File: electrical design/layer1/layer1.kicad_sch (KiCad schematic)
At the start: 76 parts, among them SW1 SW_DPDT_x2, U1 STM32F103C8T6, U2 CD74HC4067SM, U3 CD74HC4067SM

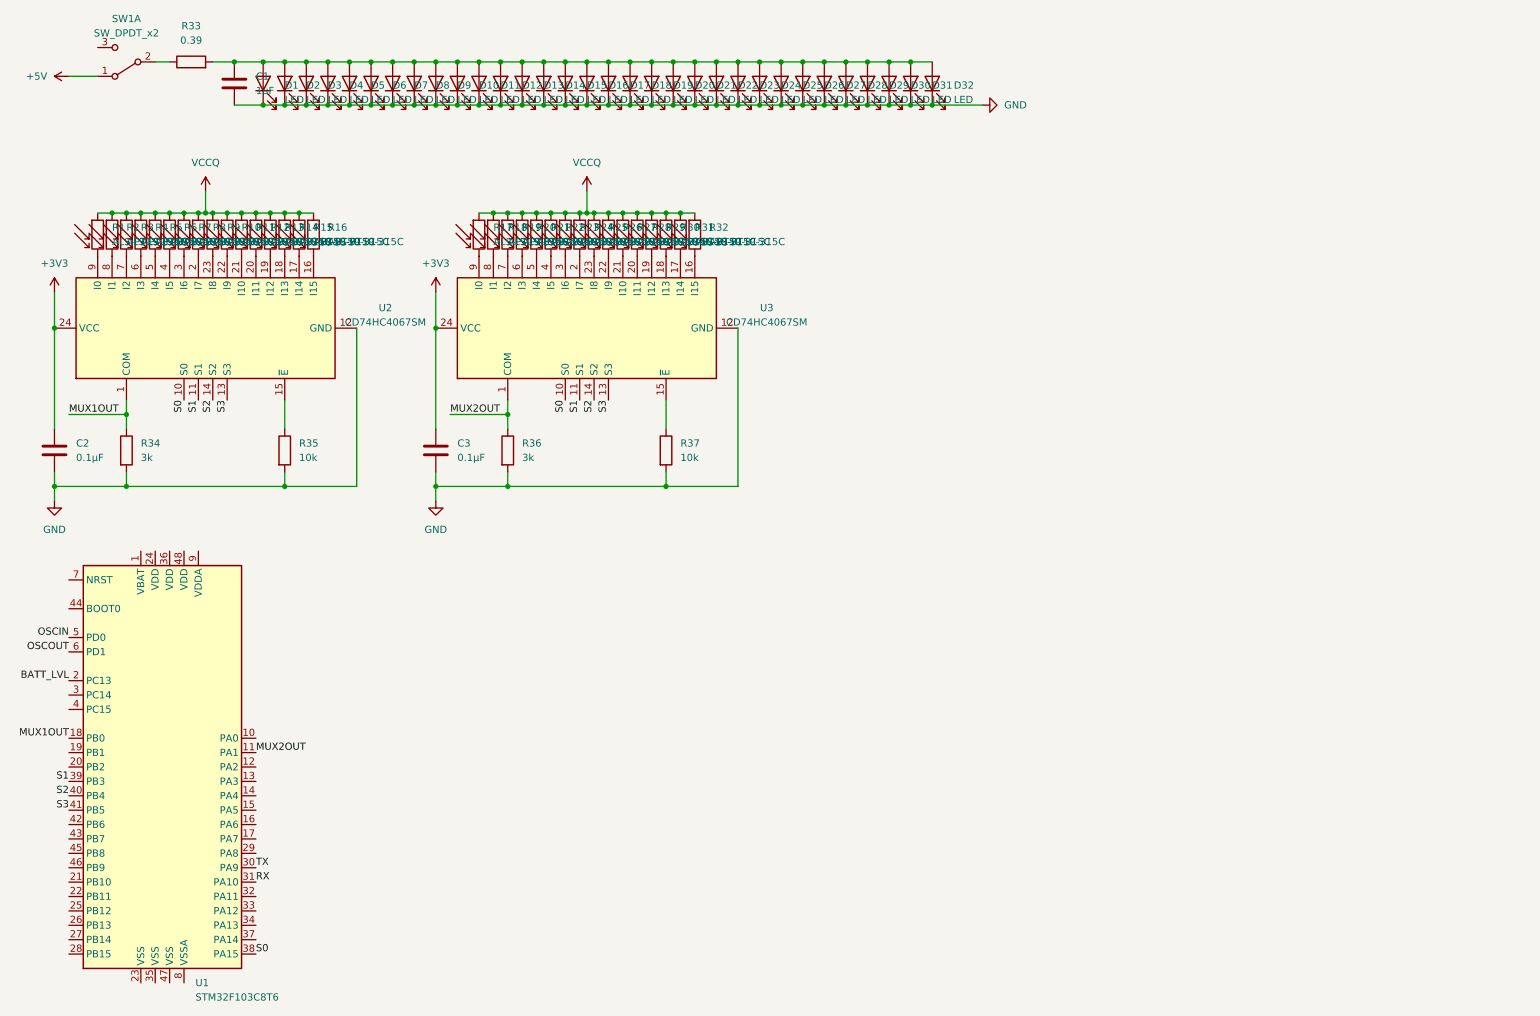
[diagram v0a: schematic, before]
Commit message: finish stm32f103c8t6 sub-circuit
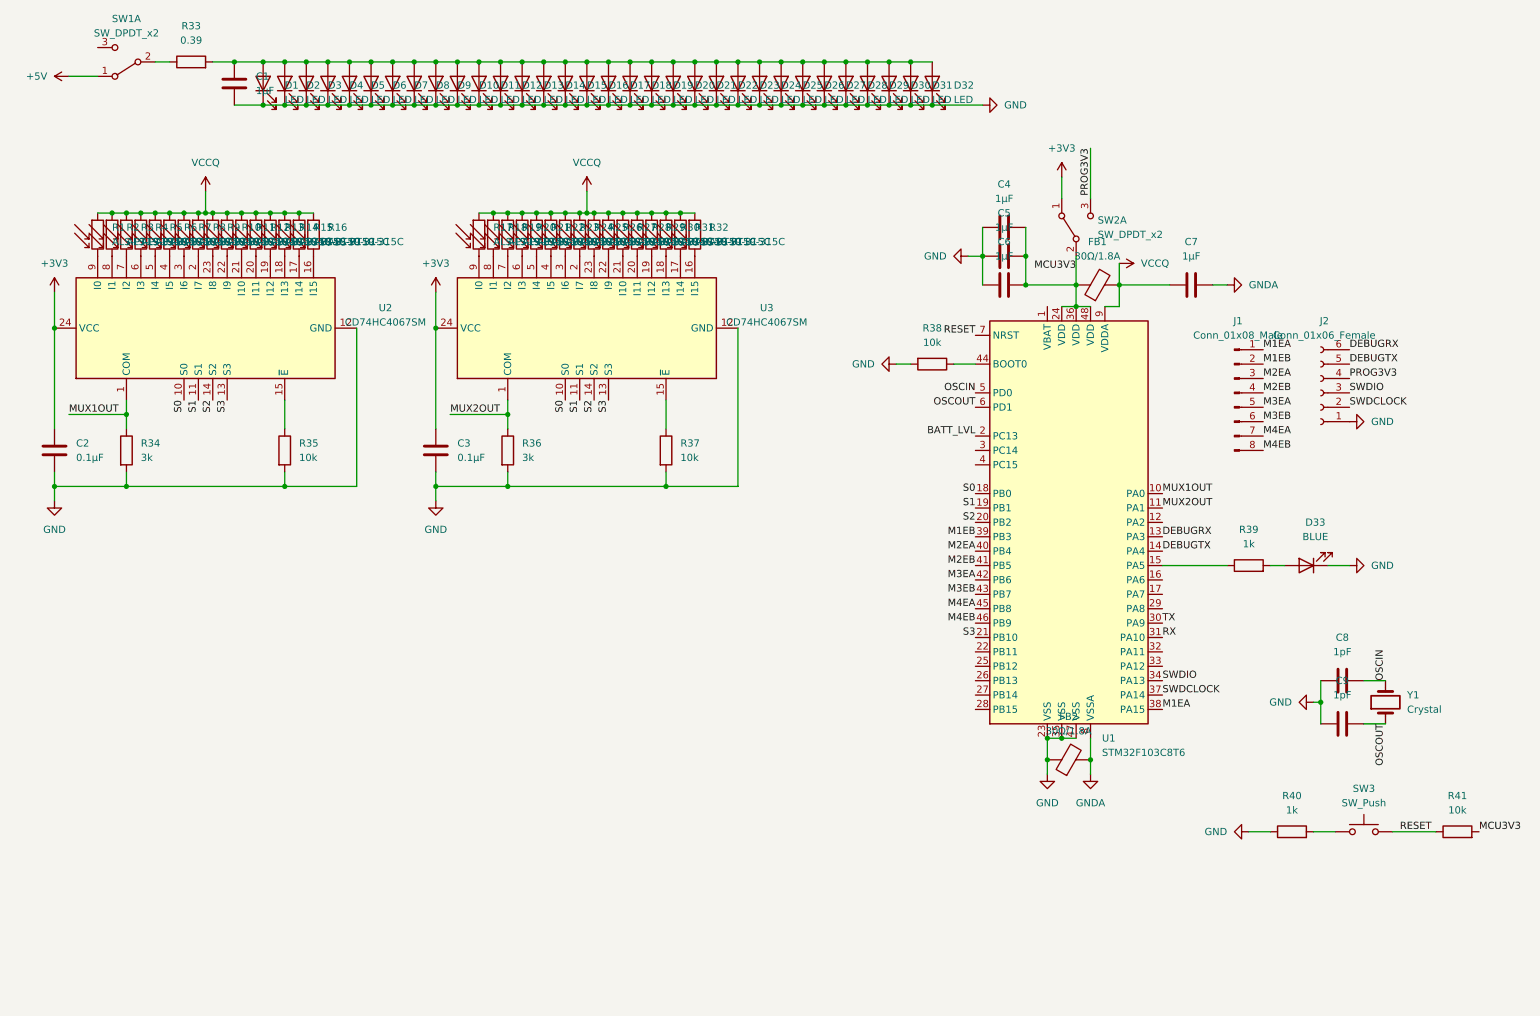
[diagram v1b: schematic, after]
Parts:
- added C4, C5, C6, C7: 1μF, symbol Device:C
- added C8, C9: 1pF, Capacitors:0603, symbol Device:C
- added D33: BLUE, symbol Device:LED
- added FB1, FB2: 30Ω/1.8A, symbol Device:FerriteBead
- added J1: Conn_01x08_Male, symbol Connector:Conn_01x08_Male
- added J2: Conn_01x06_Female, Connector_JST:JST_SH_BM06B-SRSS-TB_1x06-1MP_P1.00mm_Vertical, symbol Connector:Conn_01x06_Female
- added R38, R41: 10k, symbol Device:R
- added R39, R40: 1k, symbol Device:R
- added SW2: SW_DPDT_x2, symbol Switch:SW_DPDT_x2
- added SW3: SW_Push, symbol Switch:SW_Push
- added Y1: Crystal, Clocks:CRYSTAL-SMD-5X3.2-2PAD, symbol Device:Crystal
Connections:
- net +3V3: now also SW2.1 (A)
- net GND: now also U1.23 (VSS), U1.35 (VSS), U1.47 (VSS), C4.1, C5.1, C6.1, C8.1, C9.1, D33.1 (K), FB2.1, J2.1 (Pin_1), R38.2, R40.1
- net MUX1OUT: now also U1.10 (PA0); no longer U1.18 (PB0)
- net OSCIN: now also C8.2, Y1.2
- net OSCOUT: now also C9.2, Y1.1
- net S0: now also U1.18 (PB0); no longer U1.38 (PA15)
- net S1: now also U1.19 (PB1); no longer U1.39 (PB3)
- net S2: now also U1.20 (PB2); no longer U1.40 (PB4)
- net S3: now also U1.21 (PB10); no longer U1.41 (PB5)
- net VCCQ: now also U1.9 (VDDA), C7.1, FB1.2
- net DEBUGRX: now reaches U1.13 (PA3)
- net DEBUGRX: now also J2.6 (Pin_6)
- net DEBUGTX: now reaches U1.14 (PA4)
- net DEBUGTX: now also J2.5 (Pin_5)
- net at U1.15 (PA5): now also R39.1
- net MCU3V3: now reaches U1.24 (VDD)
- net MCU3V3: now also U1.36 (VDD), U1.48 (VDD), C4.2, C5.2, C6.2, FB1.1, R41.2, SW2.2 (B)
- net SWDIO: now reaches U1.34 (PA13)
- net SWDIO: now also J2.3 (Pin_3)
- net SWDCLOCK: now reaches U1.37 (PA14)
- net SWDCLOCK: now also J2.2 (Pin_2)
- net M3EA: now reaches U1.42 (PB6)
- net M3EA: now also J1.5 (Pin_5)
- net M3EB: now reaches U1.43 (PB7)
- net M3EB: now also J1.6 (Pin_6)
- net at U1.44 (BOOT0): now also R38.1
- net M4EA: now reaches U1.45 (PB8)
- net M4EA: now also J1.7 (Pin_7)
- net M4EB: now reaches U1.46 (PB9)
- net M4EB: now also J1.8 (Pin_8)
- net RESET: now reaches U1.7 (NRST)
- net RESET: now also R41.1, SW3.2
- net GNDA: now reaches U1.8 (VSSA)
- net GNDA: now also C7.2, FB2.2
- new net: D33.2 (A), R39.2
- new net: R40.2, SW3.1
- new net M1EA: J1.1 (Pin_1), U1.38 (PA15)
- new net M1EB: J1.2 (Pin_2), U1.39 (PB3)
- new net M2EA: J1.3 (Pin_3), U1.40 (PB4)
- new net M2EB: J1.4 (Pin_4), U1.41 (PB5)
- new net PROG3V3: J2.4 (Pin_4), SW2.3 (C)
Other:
- moved on the sheet: U1
